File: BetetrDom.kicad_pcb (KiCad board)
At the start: 4 copper layers, 155 x 83.5 mm, 86 parts, among them IC1 SiC437BED-T1-GE3, J1 XT60PW-M, J2 Raspberry_Pi_2_3, J4 XT60PW-M, Q1 PXP012-30QLJ, Q2 PXP012-30QLJ, U2 LTC4412xS6

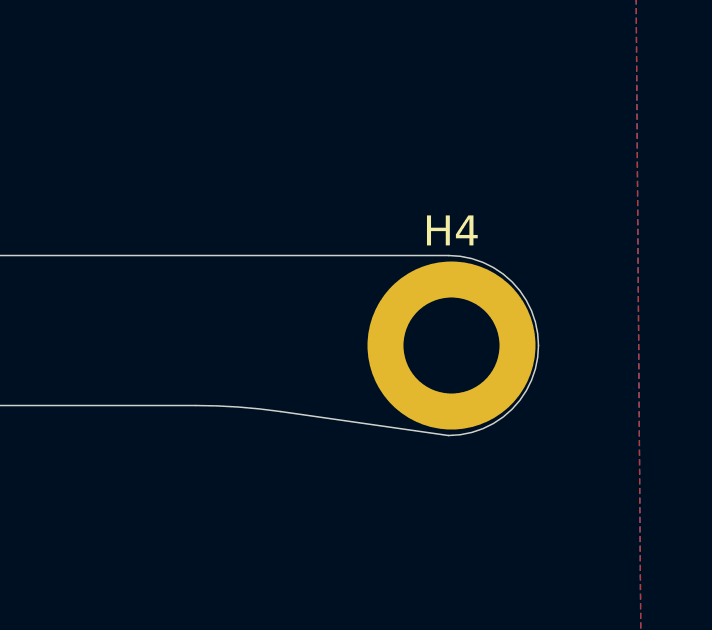
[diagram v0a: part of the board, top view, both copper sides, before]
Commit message: babs (barbara) jeng
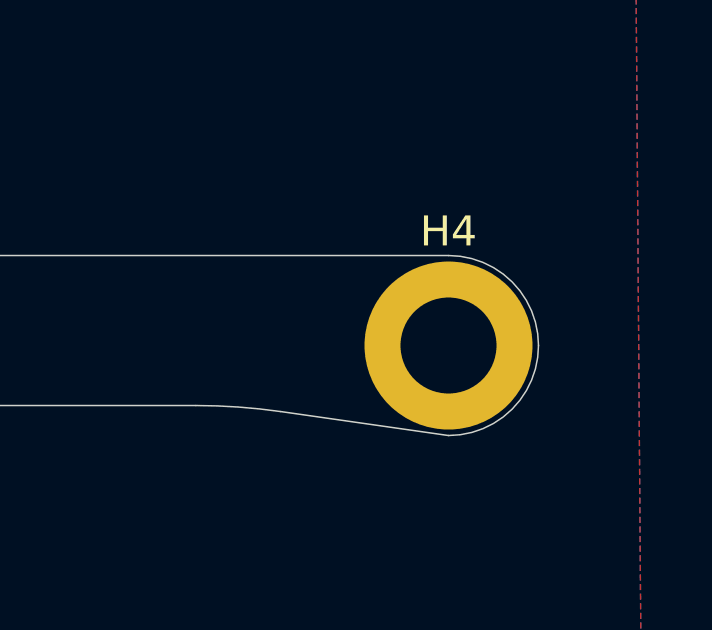
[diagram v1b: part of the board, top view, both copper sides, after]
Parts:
- moved H4 0.10 mm to (201.0, 82.0)
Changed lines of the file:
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@@
 	(footprint "MountingHole:MountingHole_3.2mm_M3_DIN965_Pad"
 		(layer "F.Cu")
-		(at 201.1 82)
+		(at 201 82)
 		(descr "Mounting Hole 3.2mm, M3, DIN965")
 		(tags "mounting hole 3.2mm m3 din965")
